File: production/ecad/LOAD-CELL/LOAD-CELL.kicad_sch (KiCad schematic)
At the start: 17 parts, among them J10 214721-0061, Q3 MMBT4403, U3 HX711

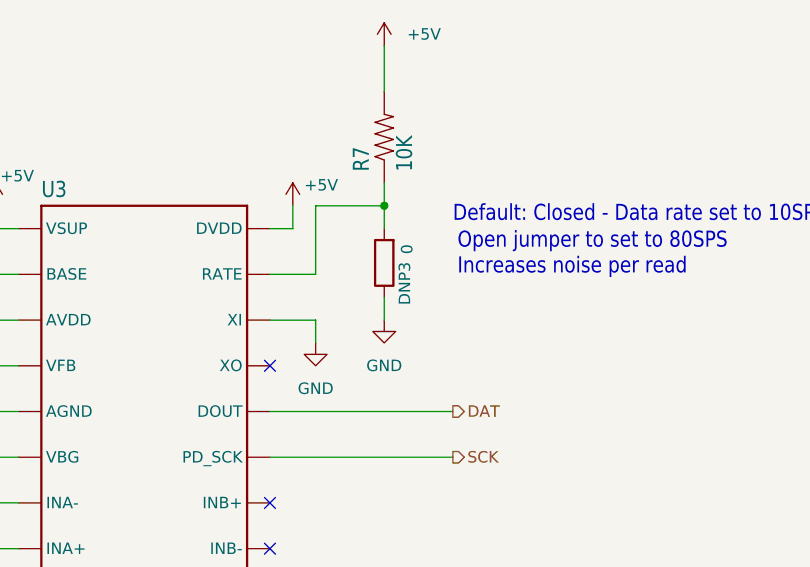
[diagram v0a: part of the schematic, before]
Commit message: david changes
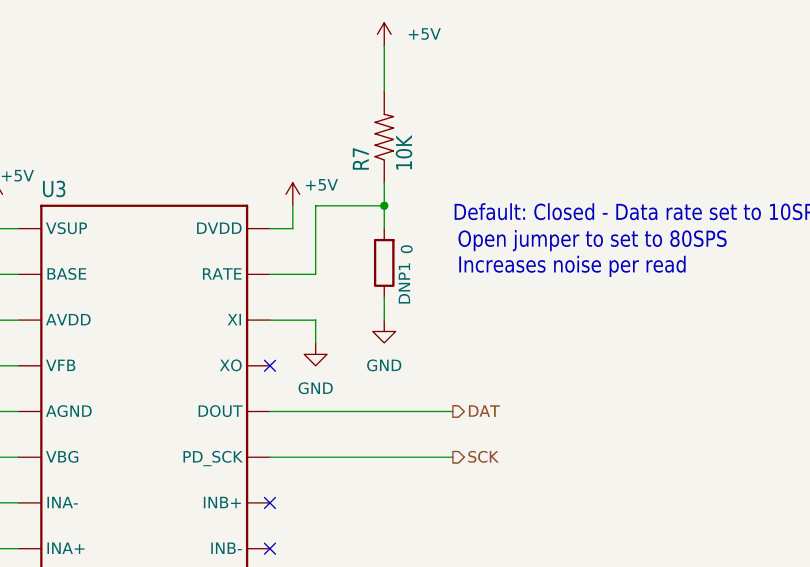
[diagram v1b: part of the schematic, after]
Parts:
- C3, C4, C6, C8, C9: footprint Load Cell and Amplifier:0603-CAP -> LoadCellFootprints:0p1uF
- C5, C7: footprint Load Cell and Amplifier:1210 -> LoadCellFootprints:10uF
- DNP1: renamed from DNP3; footprint Resistor_SMD:R_0201_0603Metric -> LoadCellFootprints:10k
- J10: footprint 2147210061 -> LoadCellFootprints:6_pos_connector
- L1: footprint Load Cell and Amplifier:0805 -> LoadCellFootprints:inductor
- Q3: footprint Load Cell and Amplifier:SOT23-3 -> LoadCellFootprints:mmbt4403
- R3: footprint Load Cell and Amplifier:0603-RES -> LoadCellFootprints:20k
- R4: footprint Load Cell and Amplifier:0603-RES -> LoadCellFootprints:8p2k
- R5, R6: footprint Load Cell and Amplifier:0603-RES -> LoadCellFootprints:100ohm
- R7: footprint Load Cell and Amplifier:0603-RES -> LoadCellFootprints:10k
- U3: footprint Load Cell and Amplifier:HX711 -> LoadCellFootprints:HX711
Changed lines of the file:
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@@
 		(on_board yes)
 		(dnp no)
-		(property "Reference" "DNP3"
+		(property "Reference" "DNP1"
 			(at 205.486 77.216 90)
 			(effects
@@
 			)
 		)
-		(property "Footprint" "Resistor_SMD:R_0201_0603Metric"
+		(property "Footprint" "LoadCellFootprints:10k"
 			(at 204.978 74.93 90)
 			(effects
@@
 			(project "Main"
 				(path "/a34d77bc-8f6a-417e-a206-3165e6c5c658/1fa8e4ec-3b8f-41b7-8956-25ba2b294586"
-					(reference "DNP3")
+					(reference "DNP1")
 					(unit 1)
 				)
@@
 			)
 		)
-		(property "Footprint" "Load Cell and Amplifier:0603-RES"
+		(property "Footprint" "LoadCellFootprints:100ohm"
 			(at 139.7 111.76 0)
 			(effects
@@
 			)
 		)
-		(property "Footprint" "Load Cell and Amplifier:1210"
+		(property "Footprint" "LoadCellFootprints:10uF"
 			(at 109.22 78.74 0)
 			(effects
@@
 			)
 		)
-		(property "Footprint" "Load Cell and Amplifier:0805"
+		(property "Footprint" "LoadCellFootprints:inductor"
 			(at 124.46 71.12 0)
 			(effects
@@
 			)
 		)
-		(property "Footprint" "Load Cell and Amplifier:HX711"
+		(property "Footprint" "LoadCellFootprints:HX711"
 			(at 177.8 88.9 0)
 			(effects
@@
 			)
 		)
-		(property "Footprint" "Load Cell and Amplifier:0603-RES"
+		(property "Footprint" "LoadCellFootprints:100ohm"
 			(at 139.7 124.46 0)
 			(effects
@@
 			)
 		)
-		(property "Footprint" "Load Cell and Amplifier:0603-CAP"
+		(property "Footprint" "LoadCellFootprints:0p1uF"
 			(at 149.86 101.6 0)
 			(effects
@@
 			)
 		)
-		(property "Footprint" "Load Cell and Amplifier:0603-CAP"
+		(property "Footprint" "LoadCellFootprints:0p1uF"
 			(at 92.71 31.75 0)
 			(effects
@@
 			)
 		)
-		(property "Footprint" "Load Cell and Amplifier:0603-CAP"
+		(property "Footprint" "LoadCellFootprints:0p1uF"
 			(at 147.32 119.38 0)
 			(effects
@@
 			)
 		)
-		(property "Footprint" "Load Cell and Amplifier:0603-RES"
+		(property "Footprint" "LoadCellFootprints:8p2k"
 			(at 137.16 93.98 0)
 			(effects
@@
 			)
 		)
-		(property "Footprint" "Load Cell and Amplifier:SOT23-3"
+		(property "Footprint" "LoadCellFootprints:mmbt4403"
 			(at 144.78 63.5 0)
 			(effects
@@
 			)
 		)
-		(property "Footprint" "2147210061"
+		(property "Footprint" "LoadCellFootprints:6_pos_connector"
 			(at 72.39 166.04 0)
 			(effects
@@
 			)
 		)
-		(property "Footprint" "Load Cell and Amplifier:0603-CAP"
+		(property "Footprint" "LoadCellFootprints:0p1uF"
 			(at 105.41 31.75 0)
 			(effects
@@
 			)
 		)
-		(property "Footprint" "Load Cell and Amplifier:0603-CAP"
+		(property "Footprint" "LoadCellFootprints:0p1uF"
 			(at 99.06 78.74 0)
 			(effects
@@
 			)
 		)
-		(property "Footprint" "Load Cell and Amplifier:0603-RES"
+		(property "Footprint" "LoadCellFootprints:10k"
 			(at 203.2 60.96 0)
 			(effects
@@
 			)
 		)
-		(property "Footprint" "Load Cell and Amplifier:1210"
+		(property "Footprint" "LoadCellFootprints:10uF"
 			(at 120.65 31.75 0)
 			(effects
@@
 			)
 		)
-		(property "Footprint" "Load Cell and Amplifier:0603-RES"
+		(property "Footprint" "LoadCellFootprints:20k"
 			(at 137.16 78.74 0)
 			(effects
